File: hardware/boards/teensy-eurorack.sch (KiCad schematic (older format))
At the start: 95 parts, among them J1 Conn_01x08, J27 Conn_01x02, J28 Conn_02x08_Odd_Even, SW1 Rotary_Encoder_Switch, SW2 Rotary_Encoder_Switch, SW3 Rotary_Encoder_Switch, U1 CS42448, U2 AD5754BREZ, U3 AD5754BREZ, U4 Teensy4.1, U5 MCP1700-2502E_SOT23, U6 AD7606BSTZ, U7 6N138

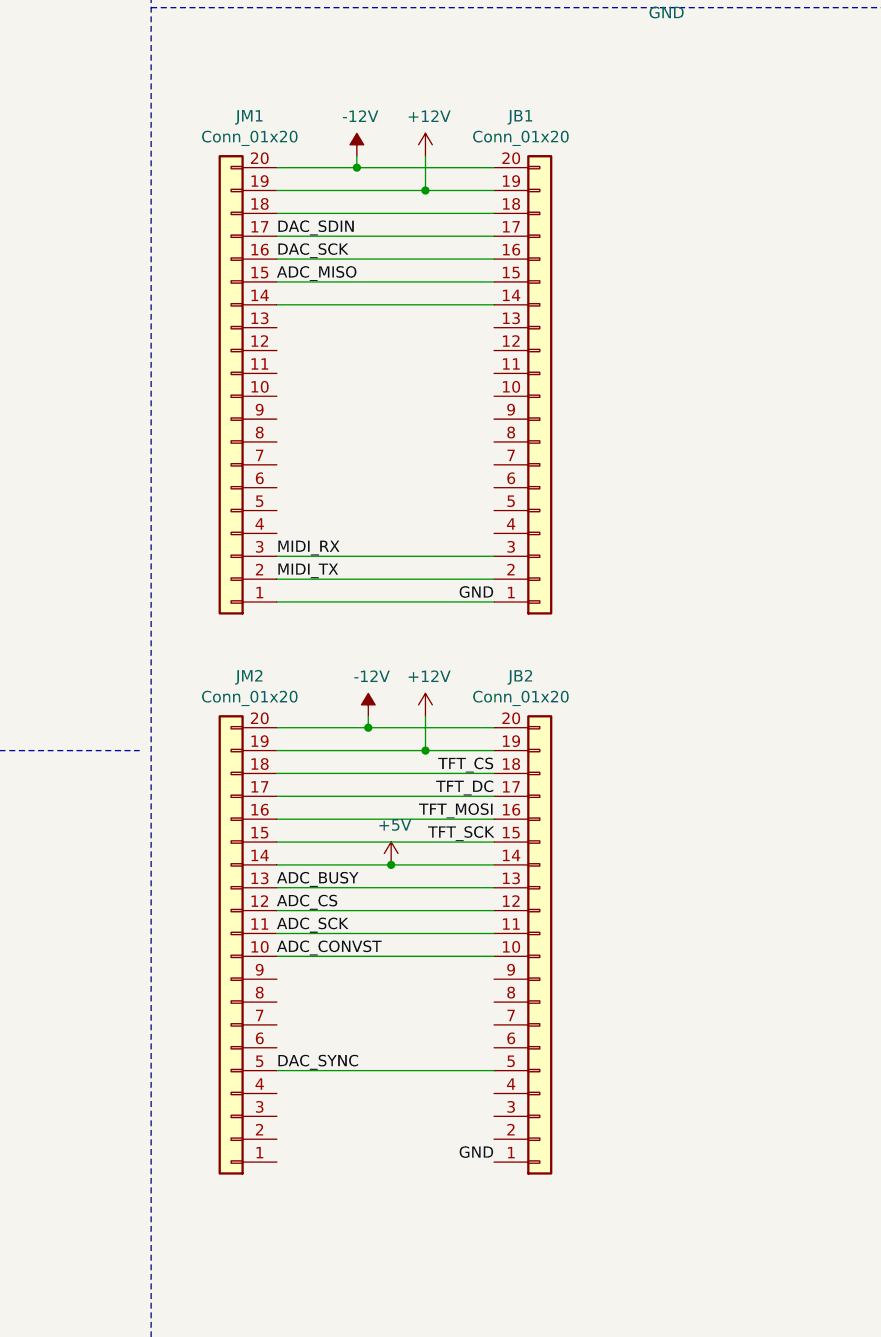
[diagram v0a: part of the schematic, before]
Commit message: slowly
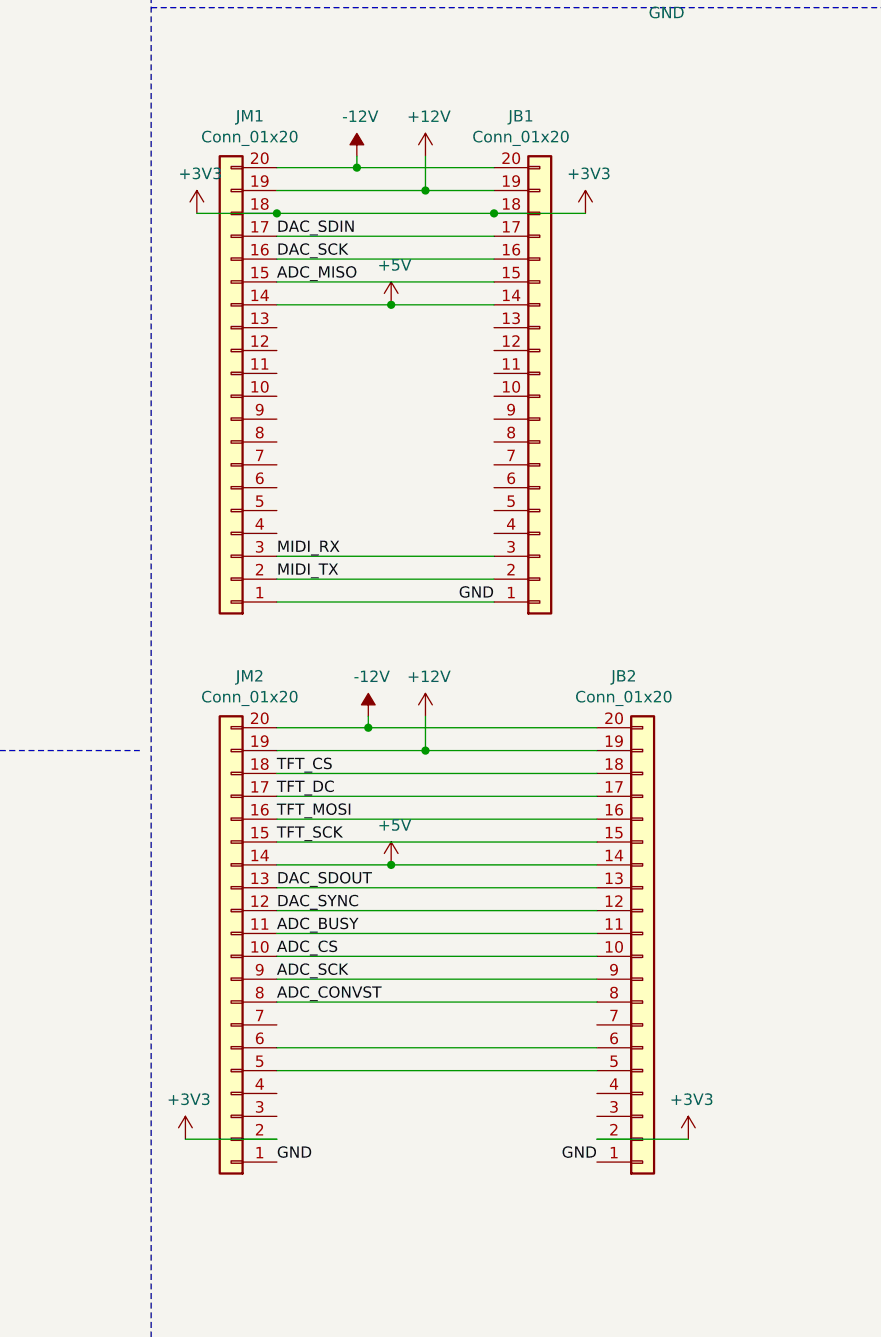
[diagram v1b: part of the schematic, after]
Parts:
- C1, C2, C3, C4: footprint Capacitor_SMD:C_0805_2012Metric -> Capacitor_THT:CP_Radial_D5.0mm_P2.50mm
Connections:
- net +3V3: now also JB1.18 (Pin_18), JB2.2 (Pin_2), JM1.18 (Pin_18), JM2.2 (Pin_2)
- net +5V: now also JB1.14 (Pin_14), JM1.14 (Pin_14)
- net ADC_BUSY: now also JB2.11 (Pin_11), JM2.11 (Pin_11); no longer JB2.13 (Pin_13), JM2.13 (Pin_13)
- net ADC_CONVST: now also JB2.8 (Pin_8), JM2.8 (Pin_8); no longer JB2.10 (Pin_10), JM2.10 (Pin_10)
- net ADC_CS: now also JB2.10 (Pin_10), JM2.10 (Pin_10); no longer JB2.12 (Pin_12), JM2.12 (Pin_12)
- net ADC_SCK: now also JB2.9 (Pin_9), JM2.9 (Pin_9); no longer JB2.11 (Pin_11), JM2.11 (Pin_11)
- net DAC_SDOUT: now also JB2.13 (Pin_13), JM2.13 (Pin_13)
- net DAC_SYNC: now also JB2.12 (Pin_12), JM2.12 (Pin_12); no longer JB2.5 (Pin_5), JM2.5 (Pin_5)
- net GND: now also JM2.1 (Pin_1)
- net at JM2.6 (Pin_6): now also JB2.6 (Pin_6)
- new net: JB2.5 (Pin_5), JM2.5 (Pin_5)
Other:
- moved on the sheet: JB2
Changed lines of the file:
@@
 Wire Wire Line
 	12000 1350 12000 1500
-Text Label 12000 1500 0    50   ~ 0
-SDA
 $Comp
 L power:GND #PWR019
@@
 F 0 "C3" H 2418 4146 50  0000 L CNN
 F 1 "4.7u" H 2418 4055 50  0000 L CNN
-F 2 "Capacitor_SMD:C_0805_2012Metric" H 2338 3950 50  0001 C CNN
+F 2 "Capacitor_THT:CP_Radial_D5.0mm_P2.50mm" H 2338 3950 50  0001 C CNN
 F 3 "~" H 2300 4100 50  0001 C CNN
 	1    2300 4100
@@
 F 0 "C2" H 2018 4146 50  0000 L CNN
 F 1 "4.7u" H 2018 4055 50  0000 L CNN
-F 2 "Capacitor_SMD:C_0805_2012Metric" H 1938 3950 50  0001 C CNN
+F 2 "Capacitor_THT:CP_Radial_D5.0mm_P2.50mm" H 1938 3950 50  0001 C CNN
 F 3 "~" H 1900 4100 50  0001 C CNN
 	1    1900 4100
@@
 F 0 "C1" H 1618 4146 50  0000 L CNN
 F 1 "4.7u" H 1618 4055 50  0000 L CNN
-F 2 "Capacitor_SMD:C_0805_2012Metric" H 1538 3950 50  0001 C CNN
+F 2 "Capacitor_THT:CP_Radial_D5.0mm_P2.50mm" H 1538 3950 50  0001 C CNN
 F 3 "~" H 1500 4100 50  0001 C CNN
 	1    1500 4100
@@
 F 0 "C4" H 2818 4146 50  0000 L CNN
 F 1 "4.7u" H 2818 4055 50  0000 L CNN
-F 2 "Capacitor_SMD:C_0805_2012Metric" H 2738 3950 50  0001 C CNN
+F 2 "Capacitor_THT:CP_Radial_D5.0mm_P2.50mm" H 2738 3950 50  0001 C CNN
 F 3 "~" H 2700 4100 50  0001 C CNN
 	1    2700 4100
@@
 L Connector_Generic:Conn_01x20 JB2
 U 1 1 5F122D19
-P 14450 6200
-F 0 "JB2" H 14368 4975 50  0000 C CNN
-F 1 "Conn_01x20" H 14368 5066 50  0000 C CNN
-F 2 "Connector_PinHeader_2.54mm:PinHeader_1x20_P2.54mm_Vertical" H 14450 6200 50  0001 C CNN
-F 3 "~" H 14450 6200 50  0001 C CNN
-	1    14450 6200
+P 14900 6200
+F 0 "JB2" H 14818 4975 50  0000 C CNN
+F 1 "Conn_01x20" H 14818 5066 50  0000 C CNN
+F 2 "Connector_PinHeader_2.54mm:PinHeader_1x20_P2.54mm_Vertical" H 14900 6200 50  0001 C CNN
+F 3 "~" H 14900 6200 50  0001 C CNN
+	1    14900 6200
 	1    0    0    1
 $EndComp
@@
 Text Label 5900 9250 0    49   ~ 0
 P4
-Text Label 14250 5500 2    49   ~ 0
+Text Label 13300 5500 0    49   ~ 0
 TFT_DC
-Text Label 14250 5400 2    49   ~ 0
+Text Label 13300 5400 0    49   ~ 0
 TFT_CS
-Text Label 14250 5700 2    49   ~ 0
+Text Label 13300 5700 0    49   ~ 0
 TFT_SCK
-Text Label 14250 5600 2    49   ~ 0
+Text Label 13300 5600 0    49   ~ 0
 TFT_MOSI
-Text Label 14250 7100 2    49   ~ 0
+Text Label 13300 7100 0    49   ~ 0
 GND
 Text Label 14250 4650 2    49   ~ 0
@@
 	13300 5300 13950 5300
 Wire Wire Line
-	13300 5400 14250 5400
+	13300 5400 14700 5400
 Wire Wire Line
-	13300 5500 14250 5500
+	13300 5500 14700 5500
 Wire Wire Line
-	13300 5700 14250 5700
+	13300 5700 14700 5700
 Wire Wire Line
 	13300 5800 13800 5800
 Wire Wire Line
-	14250 5900 13300 5900
+	14700 5900 13300 5900
 Wire Wire Line
-	14250 6000 13300 6000
+	14700 6000 13300 6000
 Wire Wire Line
 	13300 4650 14250 4650
@@
 	13300 2850 13950 2850
 Wire Wire Line
-	13300 2950 14250 2950
-Wire Wire Line
 	13300 3050 14250 3050
 Text Label 13300 4550 0    49   ~ 0
@@
 Text Label 13300 4450 0    49   ~ 0
 MIDI_RX
-Text Label 13300 5900 0    49   ~ 0
+Text Label 13300 6100 0    49   ~ 0
 ADC_BUSY
 Wire Wire Line
@@
 Wire Wire Line
 	15250 900  15300 900
-Text Label 13300 6200 0    49   ~ 0
+Text Label 13300 6400 0    49   ~ 0
 ADC_CONVST
-Text Label 13300 6100 0    49   ~ 0
+Text Label 13300 6300 0    49   ~ 0
 ADC_SCK
-Text Label 13300 6000 0    49   ~ 0
+Text Label 13300 6200 0    49   ~ 0
 ADC_CS
 Text Label 13300 3250 0    49   ~ 0
 ADC_MISO
 Wire Wire Line
-	13300 6100 14250 6100
+	13300 6100 14700 6100
 Text Label 13300 3050 0    49   ~ 0
 DAC_SDIN
@@
 DAC_SCK
 Wire Wire Line
-	13300 6200 14250 6200
+	13300 6200 14700 6200
 Connection ~ 13800 5800
 Wire Wire Line
-	13800 5800 14250 5800
+	13800 5800 14700 5800
 Wire Wire Line
-	13300 5600 14250 5600
+	13300 5600 14700 5600
 Wire Wire Line
 	13300 3150 14250 3150
@@
 	10200 13400 10200 13450
 Wire Wire Line
-	13300 3350 14250 3350
+	13300 3350 13800 3350
 Wire Wire Line
 	13300 3250 14250 3250
@@
 Connection ~ 13700 5200
 Wire Wire Line
-	13700 5200 14250 5200
+	13700 5200 14700 5200
 Wire Wire Line
 	13950 5150 13950 5300
 Connection ~ 13950 5300
 Wire Wire Line
-	13950 5300 14250 5300
-Text Label 13300 6700 0    49   ~ 0
+	13950 5300 14700 5300
+Text Label 13300 6000 0    49   ~ 0
 DAC_SYNC
 Wire Wire Line
-	13300 6700 14250 6700
+	13300 6700 14700 6700
+Text Label 13300 5900 0    49   ~ 0
+DAC_SDOUT
+Wire Wire Line
+	13300 6600 14700 6600
+Wire Wire Line
+	13300 6300 14700 6300
+Wire Wire Line
+	13300 6400 14700 6400
+Text Label 12000 1500 0    50   ~ 0
+SDA
+$Comp
+L power:+5V #PWR0154
+U 1 1 5F032E74
+P 13800 3350
+F 0 "#PWR0154" H 13800 3200 50  0001 C CNN
+F 1 "+5V" H 13815 3523 50  0000 C CNN
+F 2 "" H 13800 3350 50  0001 C CNN
+F 3 "" H 13800 3350 50  0001 C CNN
+	1    13800 3350
+	1    0    0    -1
+$EndComp
+Connection ~ 13800 3350
+Wire Wire Line
+	13800 3350 14250 3350
+$Comp
+L power:+3V3 #PWR?
+U 1 1 5F063899
+P 12900 7000
+F 0 "#PWR?" H 12900 6850 50  0001 C CNN
+F 1 "+3V3" H 12915 7173 50  0000 C CNN
+F 2 "" H 12900 7000 50  0001 C CNN
+F 3 "" H 12900 7000 50  0001 C CNN
+	1    12900 7000
+	1    0    0    -1
+$EndComp
+Text Label 14700 7100 2    49   ~ 0
+GND
+$Comp
+L power:+3V3 #PWR?
+U 1 1 5F068C2B
+P 15100 7000
+F 0 "#PWR?" H 15100 6850 50  0001 C CNN
+F 1 "+3V3" H 15115 7173 50  0000 C CNN
+F 2 "" H 15100 7000 50  0001 C CNN
+F 3 "" H 15100 7000 50  0001 C CNN
+	1    15100 7000
+	1    0    0    -1
+$EndComp
+Wire Wire Line
+	12900 7000 13300 7000
+Wire Wire Line
+	14700 7000 15100 7000
+$Comp
+L power:+3V3 #PWR?
+U 1 1 5F089478
+P 12950 2950
+F 0 "#PWR?" H 12950 2800 50  0001 C CNN
+F 1 "+3V3" H 12965 3123 50  0000 C CNN
+F 2 "" H 12950 2950 50  0001 C CNN
+F 3 "" H 12950 2950 50  0001 C CNN
+	1    12950 2950
+	1    0    0    -1
+$EndComp
+$Comp
+L power:+3V3 #PWR?
+U 1 1 5F089EA5
+P 14650 2950
+F 0 "#PWR?" H 14650 2800 50  0001 C CNN
+F 1 "+3V3" H 14665 3123 50  0000 C CNN
+F 2 "" H 14650 2950 50  0001 C CNN
+F 3 "" H 14650 2950 50  0001 C CNN
+	1    14650 2950
+	1    0    0    -1
+$EndComp
+Wire Wire Line
+	12950 2950 13300 2950
+Connection ~ 13300 2950
+Wire Wire Line
+	13300 2950 14250 2950
+Connection ~ 14250 2950
+Wire Wire Line
+	14250 2950 14650 2950
 $EndSCHEMATC
